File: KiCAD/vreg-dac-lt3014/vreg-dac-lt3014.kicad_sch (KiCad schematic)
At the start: 32 parts, among them J1 Conn_01x02, J2 Conn_01x02, J3 Conn_01x02, J4 Conn_01x05, Q1 NMOS, Q2 NMOS, SW1 SW_Push, U1 LT3014xS5, U3 INA200D, U4 AD5270

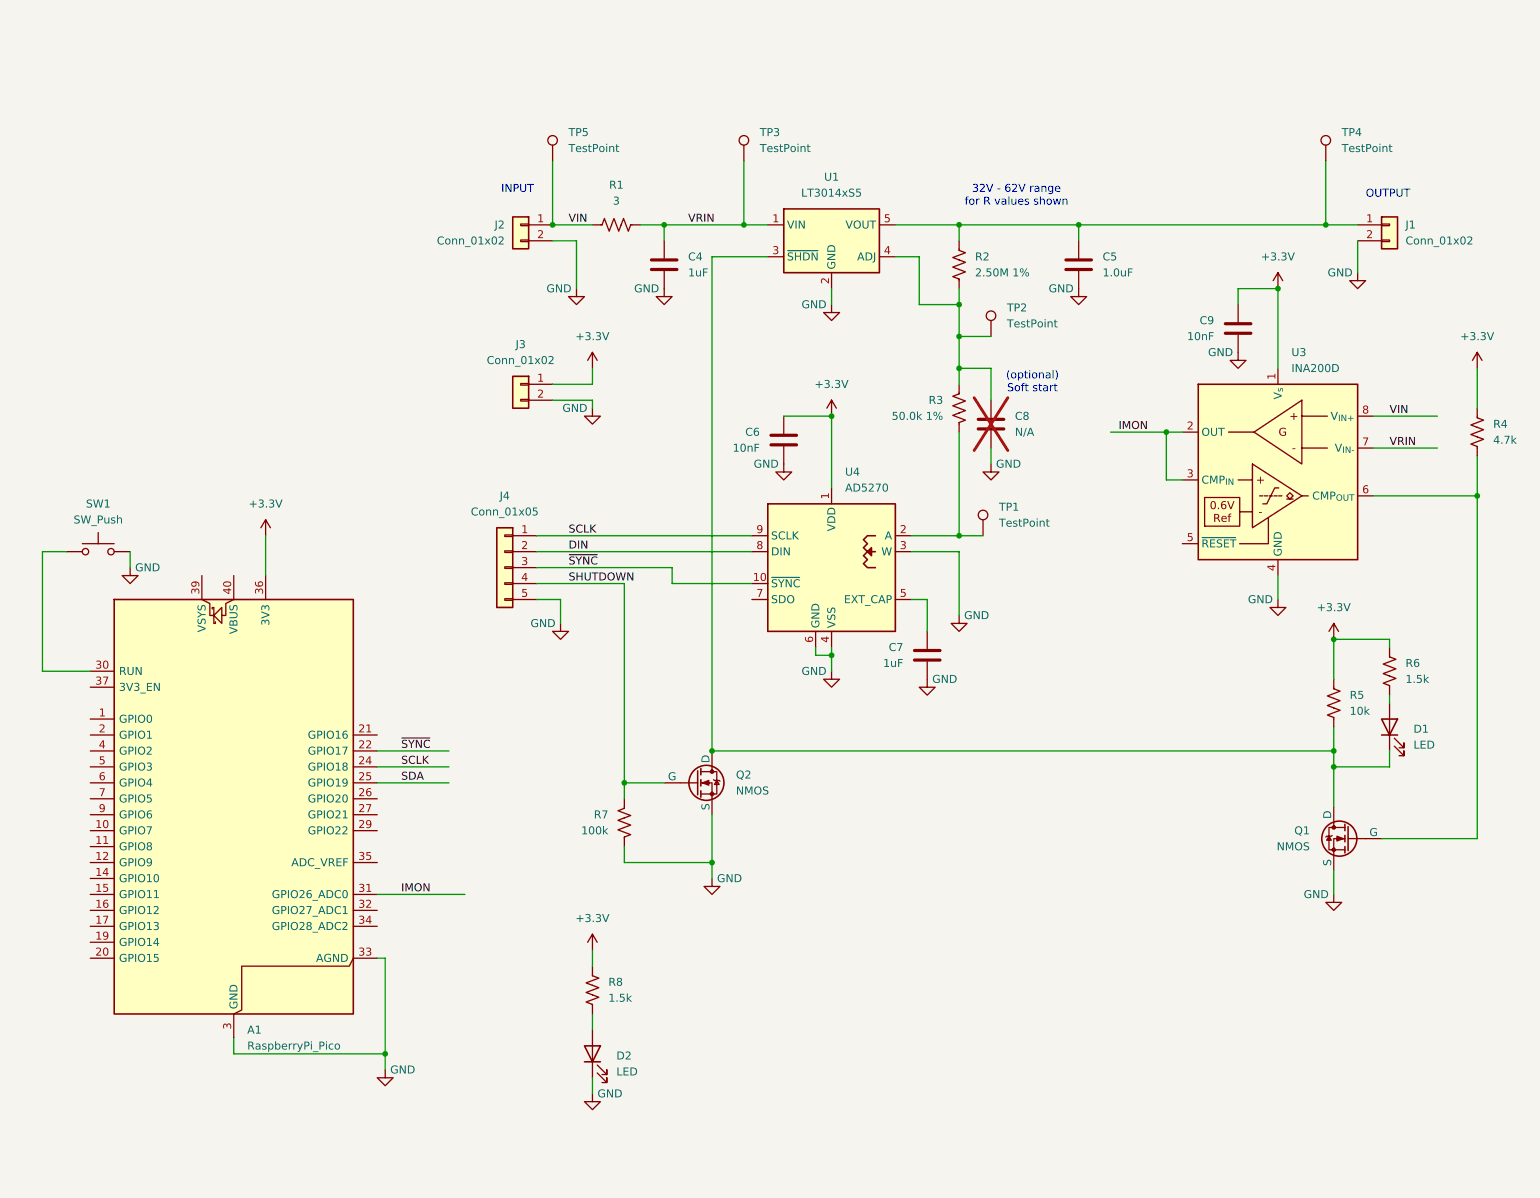
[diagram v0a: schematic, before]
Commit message: working on layout
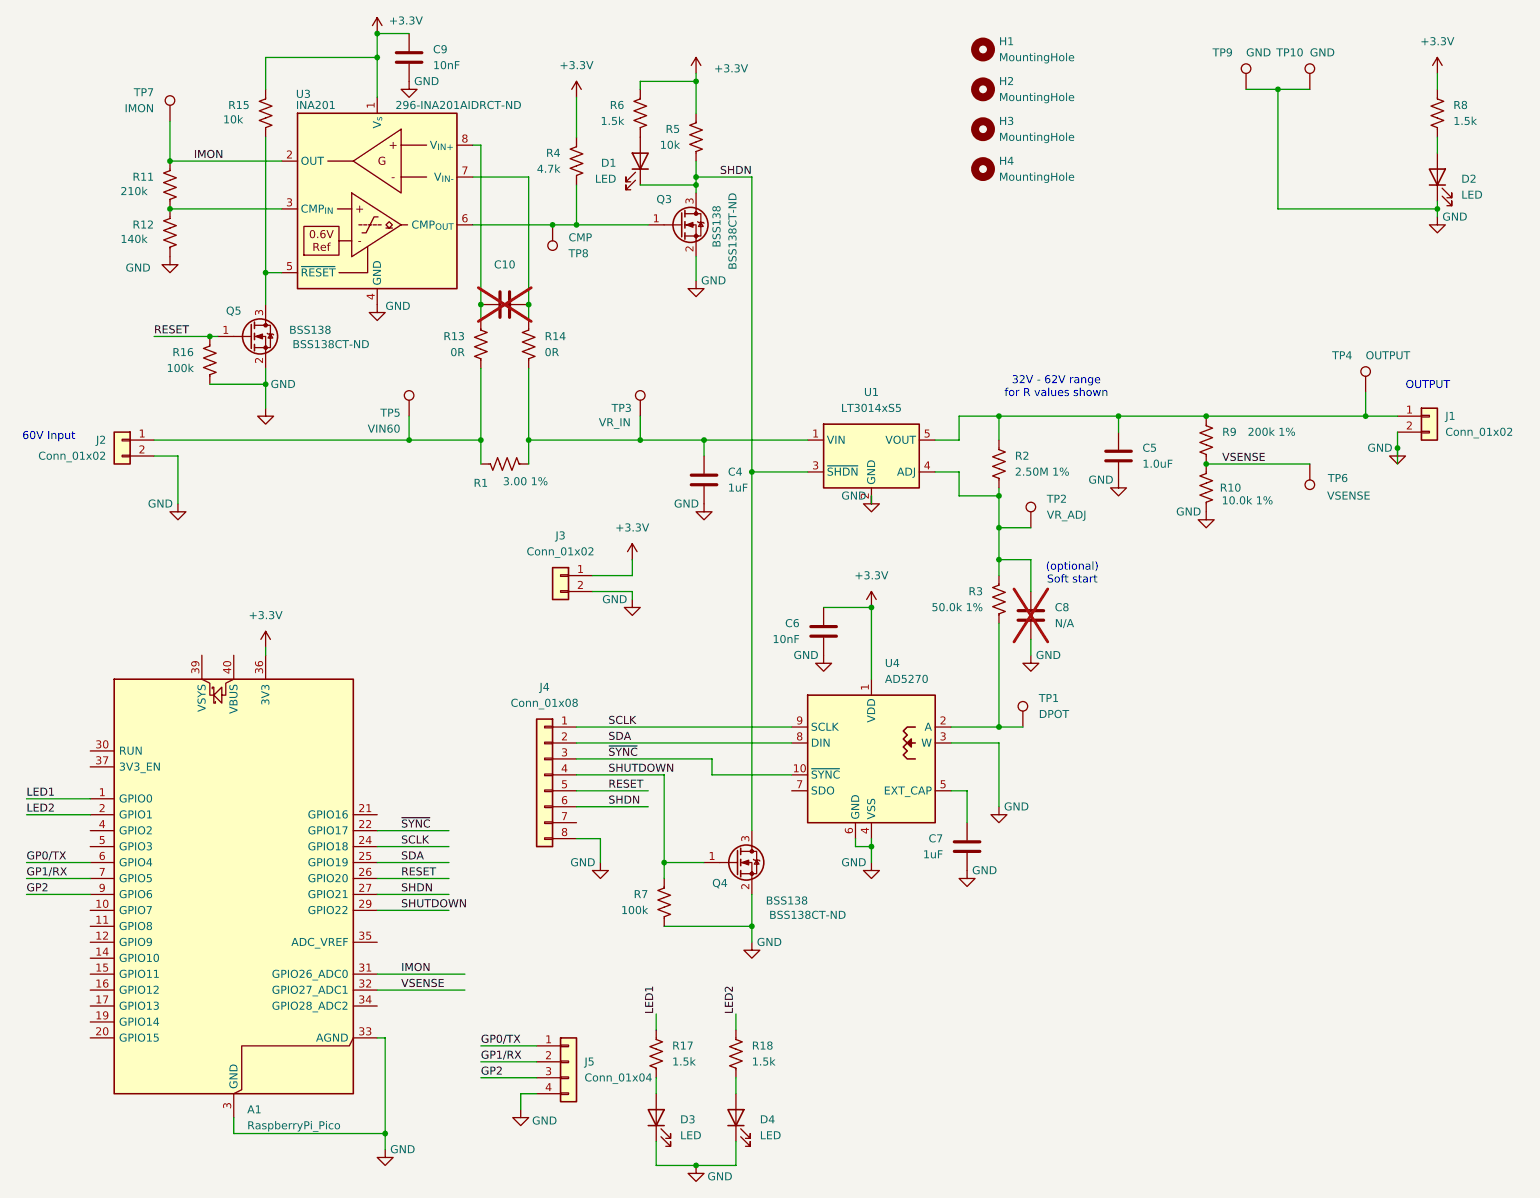
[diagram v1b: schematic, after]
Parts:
- removed J4: Conn_01x05, Connector_PinHeader_2.54mm:PinHeader_1x05_P2.54mm_Vertical, symbol Connector_Generic:Conn_01x05
- removed Q1, Q2: NMOS, Package_TO_SOT_SMD:SOT-23, symbol Simulation_SPICE:NMOS
- removed SW1: SW_Push, symbol Switch:SW_Push
- added C10: ~, Capacitor_SMD:C_0603_1608Metric_Pad1.08x0.95mm_HandSolder, symbol Device:C
- added D3, D4: LED, LED_SMD:LED_0603_1608Metric_Pad1.05x0.95mm_HandSolder, symbol Device:LED
- added H1, H2, H3, H4: MountingHole, MountingHole:MountingHole_4.3mm_M4, symbol Mechanical:MountingHole
- added J4: Conn_01x08, Connector_PinHeader_2.54mm:PinHeader_1x08_P2.54mm_Vertical, symbol Connector_Generic:Conn_01x08
- added J5: Conn_01x04, Connector_PinHeader_2.54mm:PinHeader_1x04_P2.54mm_Vertical, symbol Connector_Generic:Conn_01x04
- added Q3, Q4, Q5: BSS138, Package_TO_SOT_SMD:SOT-23, symbol Transistor_FET:BSS138
- added R10: 10.0k 1%, Resistor_SMD:R_0603_1608Metric_Pad0.98x0.95mm_HandSolder, symbol Device:R_US
- added R11: 210k, Resistor_SMD:R_0603_1608Metric_Pad0.98x0.95mm_HandSolder, symbol Device:R_US
- added R12: 140k, Resistor_SMD:R_0603_1608Metric_Pad0.98x0.95mm_HandSolder, symbol Device:R_US
- added R13, R14: 0R, Resistor_SMD:R_0603_1608Metric_Pad0.98x0.95mm_HandSolder, symbol Device:R_US
- added R15: 10k, Resistor_SMD:R_0603_1608Metric_Pad0.98x0.95mm_HandSolder, symbol Device:R_US
- added R16: 100k, Resistor_SMD:R_0603_1608Metric_Pad0.98x0.95mm_HandSolder, symbol Device:R_US
- added R17, R18: 1.5k, Resistor_SMD:R_0603_1608Metric_Pad0.98x0.95mm_HandSolder, symbol Device:R_US
- added R9: 200k 1%, Resistor_SMD:R_0603_1608Metric_Pad0.98x0.95mm_HandSolder, symbol Device:R_US
- added TP10, TP9: GND, my_tp:tp_SMT_label2, symbol Connector:TestPoint
- added TP6: VSENSE, my_tp:tp_SMT_label2, symbol Connector:TestPoint
- added TP7: IMON, my_tp:tp_SMT_label2, symbol Connector:TestPoint
- added TP8: CMP, my_tp:tp_SMT_label2, symbol Connector:TestPoint
- R1: value 3 -> 3.00 1%
- TP1: value TestPoint -> DPOT; footprint TestPoint:TestPoint_THTPad_D2.0mm_Drill1.0mm -> my_tp:tp_SMT_label2
- TP2: value TestPoint -> VR_ADJ; footprint TestPoint:TestPoint_THTPad_D2.0mm_Drill1.0mm -> my_tp:tp_SMT_label2
- TP3: value TestPoint -> VR_IN; footprint TestPoint:TestPoint_THTPad_D2.0mm_Drill1.0mm -> my_tp:tp_SMT_label2
- TP4: value TestPoint -> OUTPUT; footprint TestPoint:TestPoint_THTPad_D2.0mm_Drill1.0mm -> my_tp:tp_SMT_label2
- TP5: value TestPoint -> VIN60; footprint TestPoint:TestPoint_THTPad_D2.0mm_Drill1.0mm -> my_tp:tp_SMT_label2
- U3: value INA200D -> INA201; CatNo (none) -> 296-INA201AIDRCT-ND
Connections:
- net DIN is gone; now on net SDA: U4.8 (DIN)
- net +3.3V: now also R15.1
- net GND: now also D3.1 (K), D4.1 (K), J4.8 (Pin_8), J5.4 (Pin_4), Q3.2 (S), Q4.2 (S), Q5.2 (S), R10.2, R12.2, R16.2, TP10.1, TP9.1
- net IMON: now also R11.1, TP7.1; no longer U3.3 (CMP_{IN})
- net SCLK: now also J4.1 (Pin_1)
- net SDA: now also J4.2 (Pin_2)
- net SHUTDOWN: now also A1.29 (GPIO22), J4.4 (Pin_4), Q4.1 (G)
- net ~{SYNC}: now also J4.3 (Pin_3)
- net at C5.1, J1.1 (Pin_1), R2.1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: now also R9.1
- net SHDN: now reaches D1.1 (K), R5.2, U1.3 (~{SHDN})
- net SHDN: now also A1.27 (GPIO21), J4.6 (Pin_6), Q3.3 (D), Q4.3 (D)
- net at U3.5 (~{RESET}): now also Q5.3 (D), R15.2
- net at R4.2, U3.6 (CMP_{OUT}): now also Q3.1 (G), TP8.1
- net LED1: now reaches A1.1 (GPIO0)
- net LED1: now also R17.1
- net LED2: now reaches A1.2 (GPIO1)
- net LED2: now also R18.1
- net RESET: now reaches A1.26 (GPIO20)
- net RESET: now also J4.5 (Pin_5), Q5.1 (G), R16.1
- net VSENSE: now reaches A1.32 (GPIO27_ADC1)
- net VSENSE: now also R10.1, R9.2, TP6.1
- net GP0/TX: now reaches A1.6 (GPIO4)
- net GP0/TX: now also J5.1 (Pin_1)
- net GP1/RX: now reaches A1.7 (GPIO5)
- net GP1/RX: now also J5.2 (Pin_2)
- net GP2: now reaches A1.9 (GPIO6)
- net GP2: now also J5.3 (Pin_3)
- net VIN: no longer names the net of J2.1 (Pin_1), R1.1, TP5.1
- net VIN: now also R13.2; no longer U3.8 (V_{IN+})
- net VRIN: no longer names the net of C4.1, R1.2, TP3.1, U1.1 (VIN)
- net VRIN: now also R14.2; no longer U3.7 (V_{IN-})
- new net: R11.2, R12.1, U3.3 (CMP_{IN})
- new net: C10.2, R14.1, U3.7 (V_{IN-})
- new net: C10.1, R13.1, U3.8 (V_{IN+})
- new net: D3.2 (A), R17.2
- new net: D4.2 (A), R18.2
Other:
- note added: "60V Input"
- note removed: "INPUT"
- moved on the sheet: A1, C4, C5, C6, C7, C8, C9, D1, D2, J1, J2, J3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
